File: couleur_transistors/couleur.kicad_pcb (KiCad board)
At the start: 2 copper layers, 13.7 x 33.5 mm, 17 parts, among them P1 CONN_02X03, P2 Mounting, Q1 Q_PNP_BEC, Q2 Q_PNP_BEC, Q3 Q_PNP_BEC, U1 S4282-51

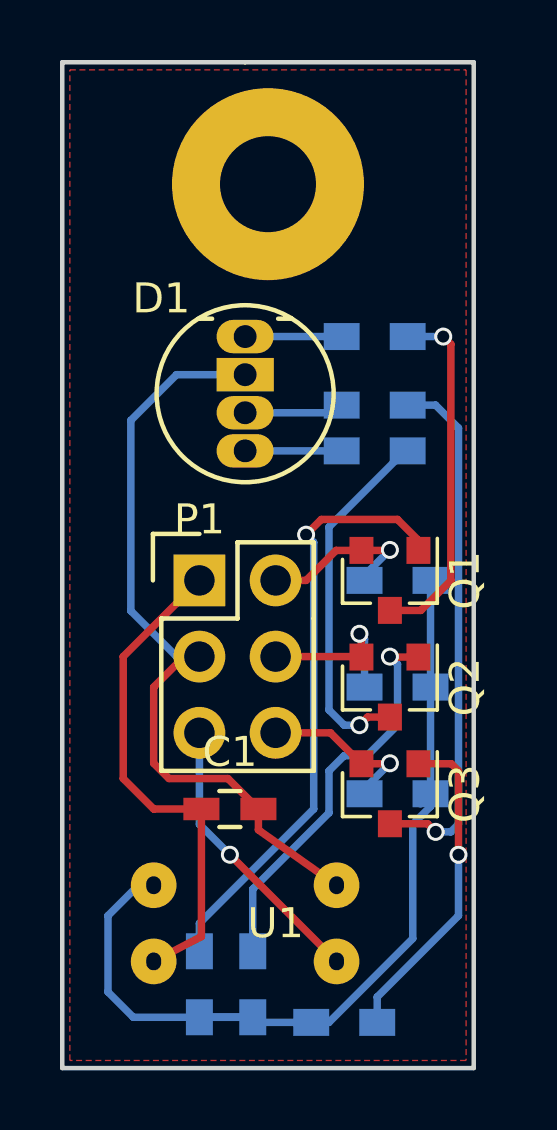
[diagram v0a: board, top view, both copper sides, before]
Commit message: Couleur
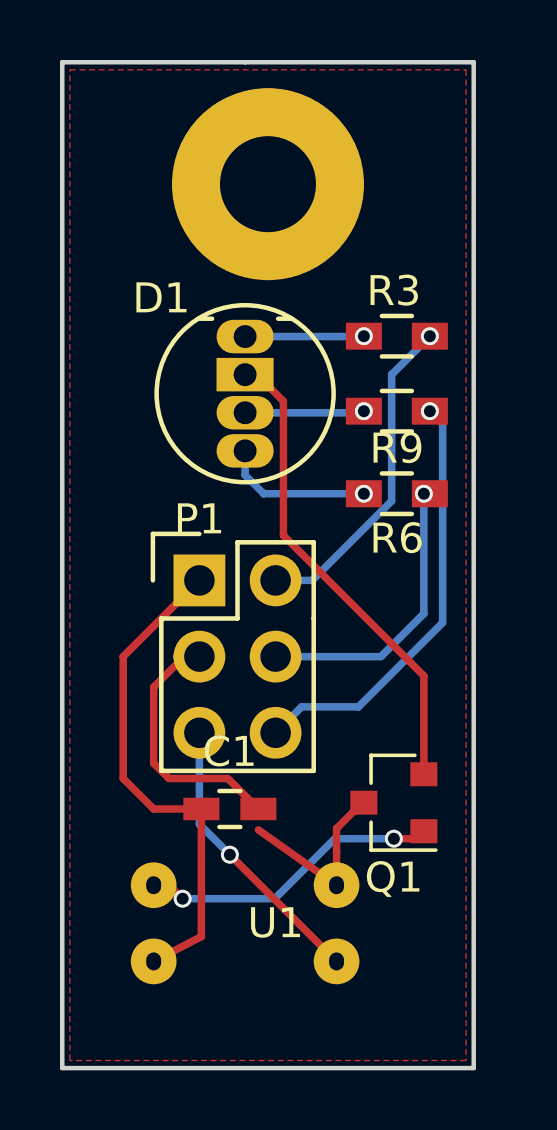
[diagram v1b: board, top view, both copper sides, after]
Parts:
- removed Q2, Q3: Q_PNP_BEC, TO_SOT_Packages_SMD:SOT-23
- removed R1, R4, R7: 0, Resistors_SMD:R_0603_HandSoldering
- removed R2, R5, R8: 100, Resistors_SMD:R_0603_HandSoldering
- R3, R6, R9: moved to F.Cu
- moved Q1 7.41 mm to (182.2, 111.5), turned to 180 degrees
- moved R6 1.61 mm to (182.3, 101.2)
- moved R9 0.77 mm to (182.3, 98.5)
- moved R3 0.74 mm to (182.3, 96.0)
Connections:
- D1 pad 2: GND -> Net-(D1-Pad2)
- Q1 pad 1: Net-(Q1-Pad1) -> CATH
- Q1 pad 2: RED -> Net-(D1-Pad2)
- Q1 pad 3: Net-(Q1-Pad3) -> GND
- R3 pad 1: Net-(Q1-Pad3) -> RED
- R6 pad 1: Net-(Q2-Pad3) -> GREEN
- R9 pad 1: Net-(Q3-Pad3) -> BLUE
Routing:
- net CATH: track 31.3 -> 10.6 mm, vias 0 -> 2
- net Net-(Q1-Pad1): track 20.1 -> 0.00 mm, vias 1 -> 0
- net Net-(Q3-Pad3): track 17.7 -> 0.00 mm, vias 1 -> 0
- net Net-(D1-Pad2): track 0.00 -> 16.0 mm
- net Net-(Q2-Pad1): track 13.3 -> 0.00 mm, vias 1 -> 0
- net Net-(Q2-Pad3): track 12.1 -> 0.00 mm, vias 1 -> 0
- net Net-(Q1-Pad3): track 11.9 -> 0.00 mm, vias 1 -> 0
- net Net-(Q3-Pad1): track 10.9 -> 0.00 mm, vias 1 -> 0
- net GND: track 26.2 -> 15.7 mm
- net BLUE: track 5.61 -> 14.3 mm
- net RED: track 5.85 -> 11.0 mm
- net GREEN: track 5.53 -> 9.82 mm
- net Net-(D1-Pad4): track 3.47 -> 5.02 mm, vias 0 -> 1
- net Net-(D1-Pad1): track 3.22 -> 3.98 mm, vias 0 -> 1
- net Net-(D1-Pad3): track 3.32 -> 4.05 mm, vias 0 -> 1
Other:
- board text added: "R G B"
- board text removed: "B"
- board text removed: "G"
- board text removed: "R"
